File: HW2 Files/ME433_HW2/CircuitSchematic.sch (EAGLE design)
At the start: 15 parts

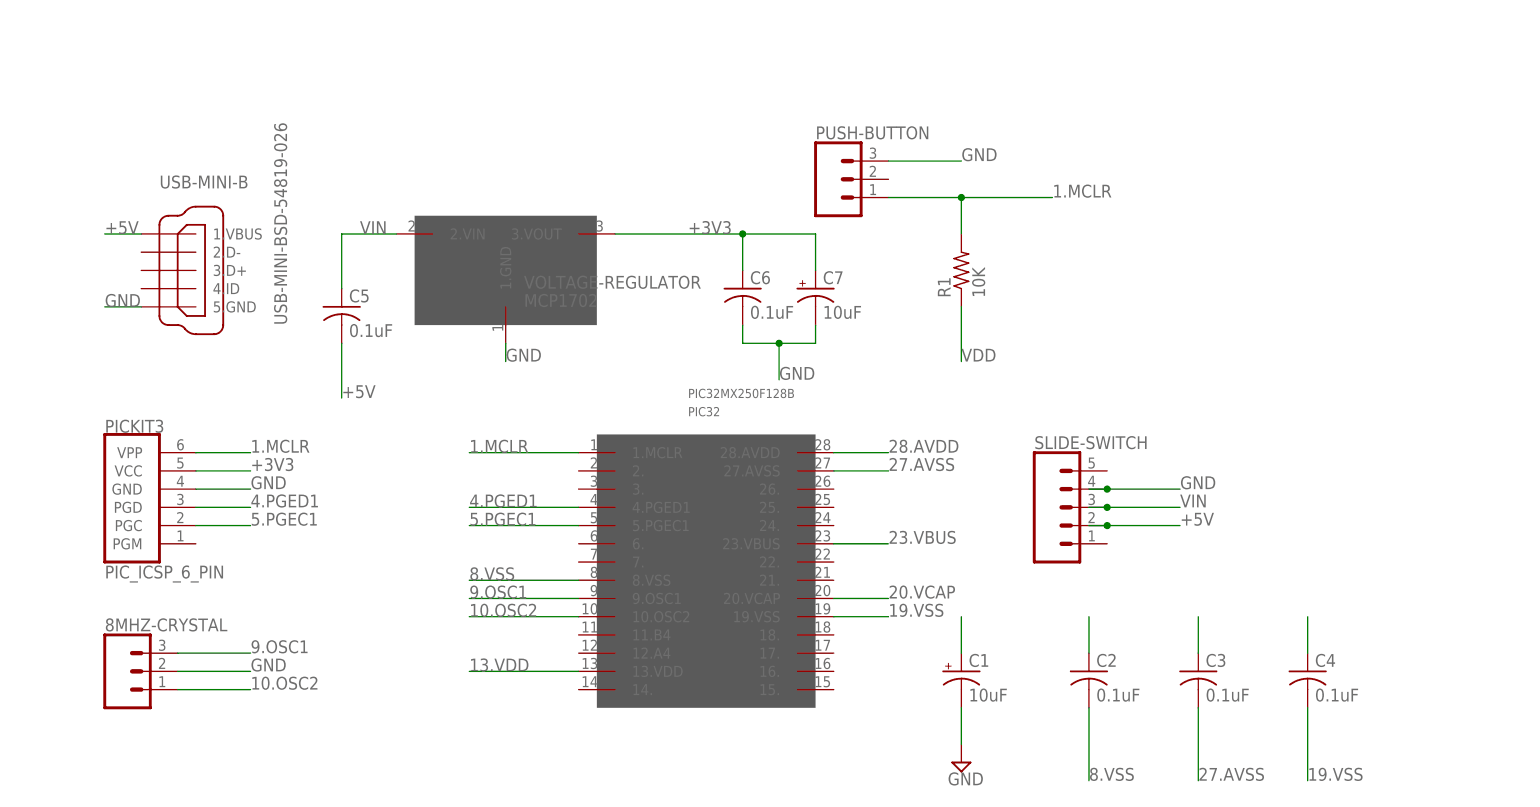
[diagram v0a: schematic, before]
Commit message: Completed schematic
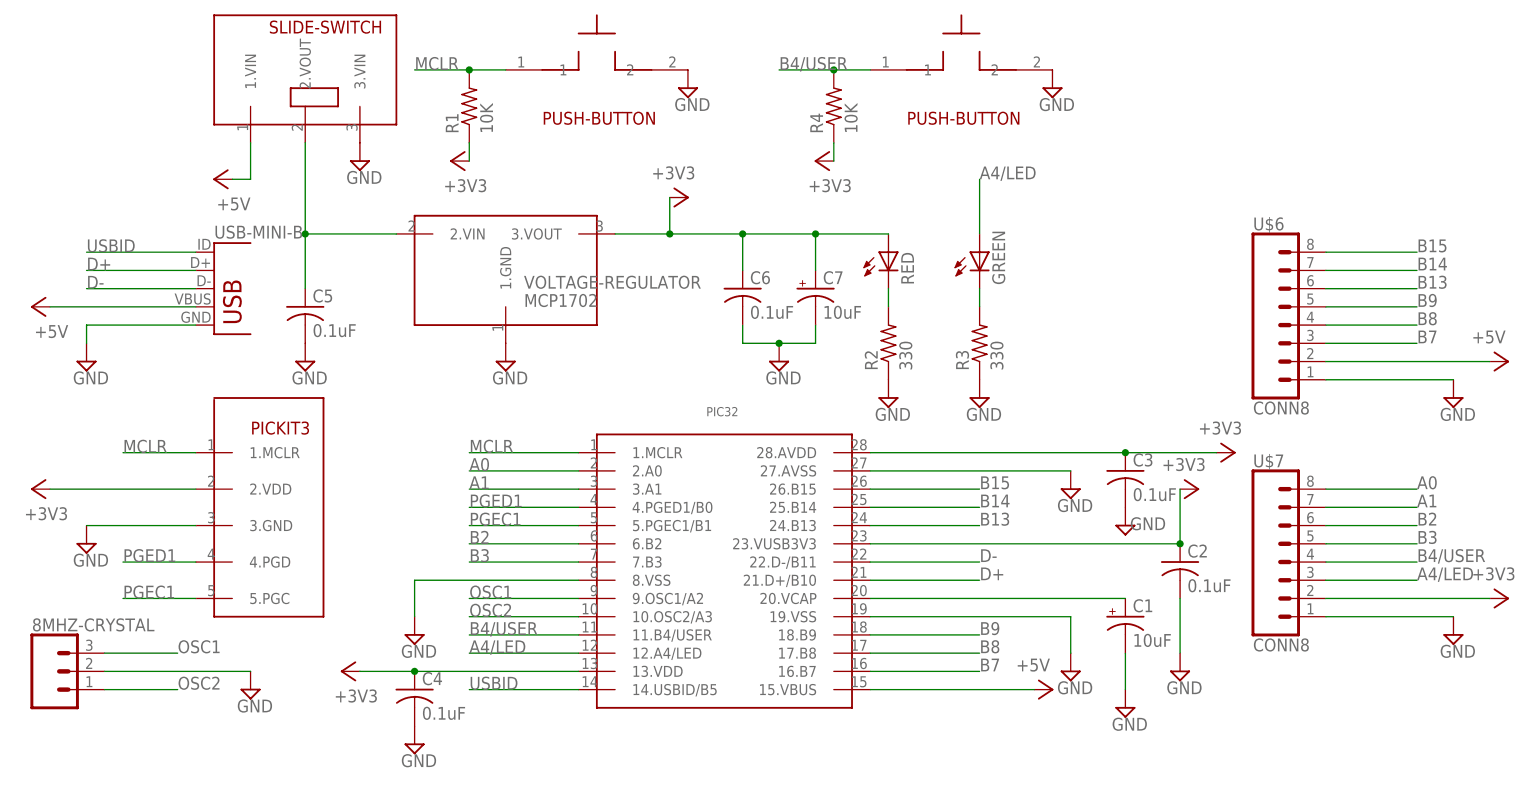
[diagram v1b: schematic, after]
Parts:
- removed PIC32MX250F128B: PIC32, ME433:PIC32
- removed PICKIT3: PIC_ICSP_6_PIN, SparkFun-Connectors:PIC_ICSP_6_PIN
- removed PUSH-BUTTON: (no value), SparkFun-Connectors:CONN_03
- removed SLIDE-SWITCH: (no value), SparkFun-Connectors:CONN_05JST-VERT
- added GREEN, RED: (no value), led:LED3MM
- added R2, R3: 330, resistor:R-US_0207/10
- added R4: 10K, resistor:R-US_0207/10
- added U$1: SLIDE-SWITCH, ME433:SLIDE-SWITCH
- added U$2, U$3: PUSH-BUTTON, ME433:PUSH-BUTTON
- added U$4: PIC32, ME433:PIC32
- added U$5: PICKIT3, ME433:PICKIT3
- added U$6, U$7: CONN8, ME433:CONN8
- USB-MINI-B: value USB-MINI-BSD-54819-026 -> USB-MB-H; device ME433:USB-MINI-BSD-54819-026 -> ME433:USB-MB-H
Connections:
- removed net 1.MCLR: PIC32MX250F128B.1.MCLR, PICKIT3.VPP, PUSH-BUTTON.1, R1.2
- removed net 10.OSC2: 8MHZ-CRYSTAL.1, PIC32MX250F128B.10.OSC2
- removed net 13.VDD: C2.1, PIC32MX250F128B.13.VDD
- removed net 19.VSS: C4.2, PIC32MX250F128B.19.VSS
- removed net 20.VCAP: C1.+, PIC32MX250F128B.20.VCAP
- removed net 23.VBUS: C4.1, PIC32MX250F128B.23.VBUS
- removed net 27.AVSS: C3.2, PIC32MX250F128B.27.AVSS
- removed net 28.AVDD: C3.1, PIC32MX250F128B.28.AVDD
- removed net 4.PGED1: PIC32MX250F128B.4.PGED1, PICKIT3.PGD
- removed net 5.PGEC1: PIC32MX250F128B.5.PGEC1, PICKIT3.PGC
- removed net 8.VSS: C2.2, PIC32MX250F128B.8.VSS
- removed net 9.OSC1: 8MHZ-CRYSTAL.3, PIC32MX250F128B.9.OSC1
- removed net VDD: R1.1
- removed net VIN: C5.1, SLIDE-SWITCH.3, VOLTAGE-REGULATOR.2.VIN
- new net A0: U$4.2.A0, U$7.8
- new net A1: U$4.3.A1, U$7.7
- new net A4/LED: GREEN.A, U$4.12.A4/LED, U$7.3
- new net B13: U$4.24.B13, U$6.6
- new net B14: U$4.25.B14, U$6.7
- new net B15: U$4.26.B15, U$6.8
- new net B2: U$4.6.B2, U$7.6
- new net B3: U$4.7.B3, U$7.5
- new net B4/USER: R4.2, U$3.1, U$4.11.B4/USER, U$7.4
- new net B7: U$4.16.B7, U$6.3
- new net B8: U$4.17.B8, U$6.4
- new net B9: U$4.18.B9, U$6.5
- new net D+: U$4.21.D+/B10, USB-MINI-B.D+
- new net D-: U$4.22.D-/B11, USB-MINI-B.D-
- new net MCLR: R1.2, U$2.1, U$4.1.MCLR, U$5.1.MCLR
- new net N$1: C1.+, U$4.20.VCAP
- new net N$2: R2.2, RED.C
- new net N$3: GREEN.C, R3.2
- new net N$4: C5.1, U$1.2.VOUT, VOLTAGE-REGULATOR.2.VIN
- new net OSC1: 8MHZ-CRYSTAL.3, U$4.9.OSC1/A2
- new net OSC2: 8MHZ-CRYSTAL.1, U$4.10.OSC2/A3
- new net PGEC1: U$4.5.PGEC1/B1, U$5.5.PGC
- new net PGED1: U$4.4.PGED1/B0, U$5.4.PGD
- new net USBID: U$4.14.USBID/B5, USB-MINI-B.ID
- net +3V3: now also C2.1, C3.1, C4.1, R1.1, R4.1, RED.A, U$4.13.VDD, U$4.23.VUSB3V3, U$4.28.AVDD, U$5.2.VDD, U$7.2; no longer PICKIT3.VCC
- net +5V: now also U$1.1.VIN, U$4.15.VBUS, U$6.2, USB-MINI-B.VBUS; no longer C5.2, SLIDE-SWITCH.2, USB-MINI-B>NAME.1.VBUS
- net GND: now also C2.2, C3.2, C4.2, C5.2, R2.1, R3.1, U$1.3.VIN, U$2.2, U$3.2, U$4.19.VSS, U$4.27.AVSS, U$4.8.VSS, U$5.3.GND, U$6.1, U$7.1, USB-MINI-B.GND; no longer PICKIT3.GND, PUSH-BUTTON.3, SLIDE-SWITCH.4, USB-MINI-B>NAME.5.GND
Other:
- moved on the sheet: 8MHZ-CRYSTAL, C1, C2, C3, C4, C5, R1
